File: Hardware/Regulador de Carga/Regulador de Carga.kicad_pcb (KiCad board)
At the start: 2 copper layers, 56 x 30 mm, 17 parts, among them Q1 2N3904

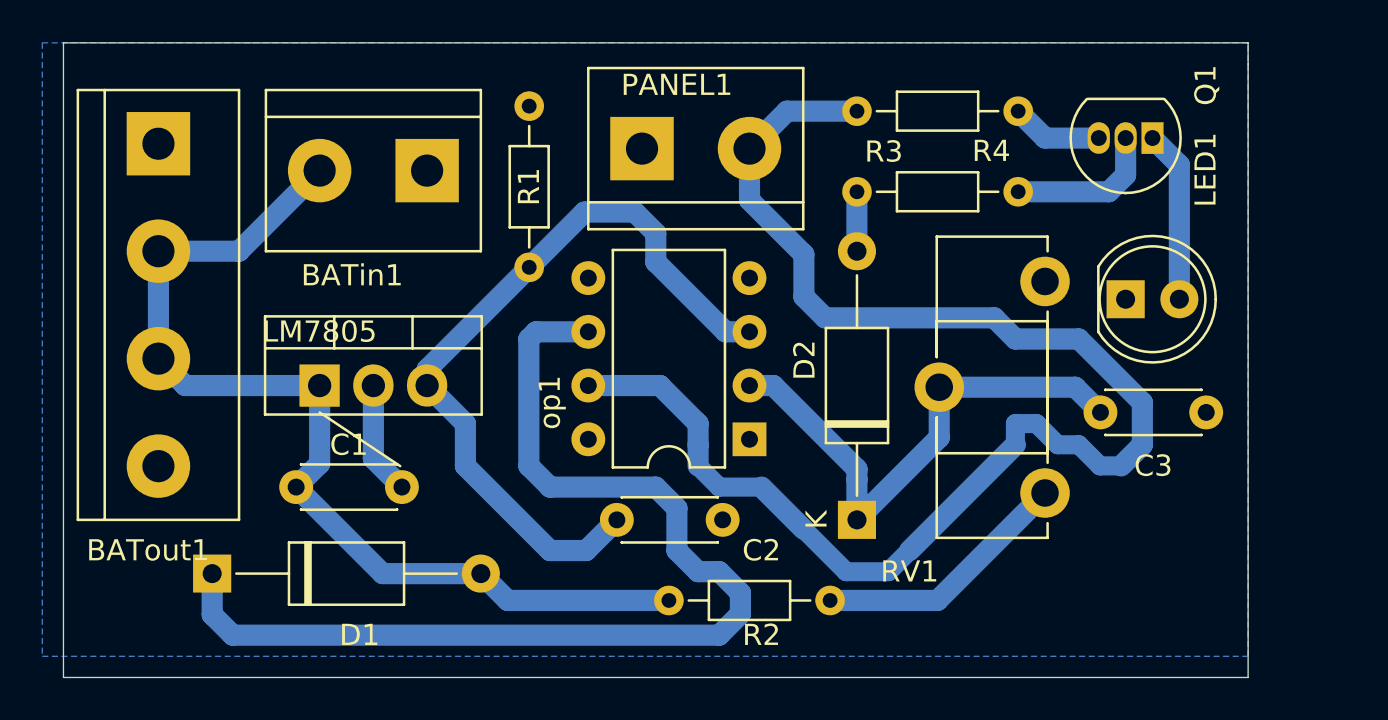
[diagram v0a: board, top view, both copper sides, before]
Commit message: PCB regulador de carga
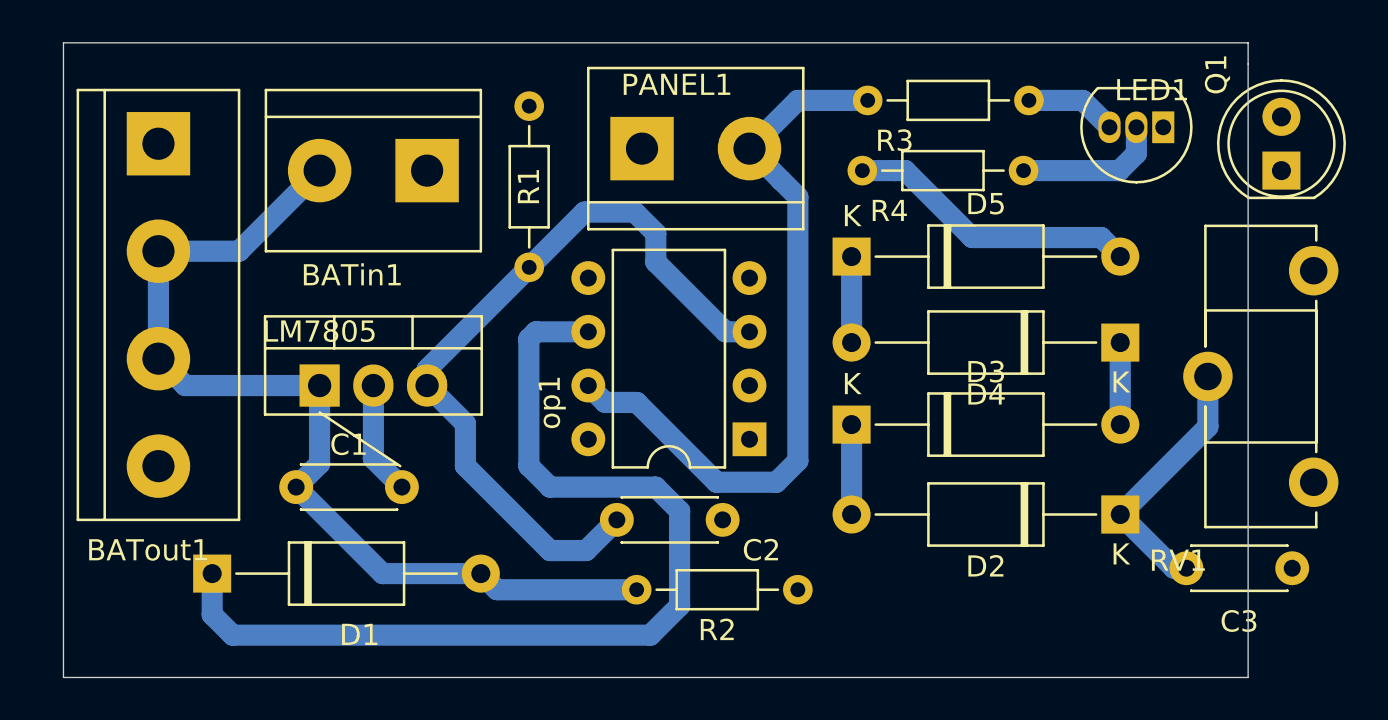
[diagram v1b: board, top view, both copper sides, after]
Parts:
- added D3: DIODE, Diode_THT:D_A-405_P12.70mm_Horizontal, F.Cu at (143.3, 78.0)
- added D4: DIODE, Diode_THT:D_A-405_P12.70mm_Horizontal, F.Cu at (156.0, 74.2)
- added D5: DIODE, Diode_THT:D_A-405_P12.70mm_Horizontal, F.Cu at (143.3, 70.1)
- D2: value D_Zener -> DIODE
- R3: value 1K -> 220
- R4: value 0K -> 220
- moved RV1 12.7 mm to (165.1, 80.8)
- moved D2 12.4 mm to (156.0, 82.3), turned to 180 degrees
- moved LED1 9.55 mm to (163.6, 66.0), turned to 90 degrees
- moved C3 8.41 mm to (164.1, 84.8)
- moved R4 7.94 mm to (151.4, 66.0), turned to 180 degrees
- moved R2 1.61 mm to (140.7, 85.9)
- moved Q1 0.72 mm to (158.0, 64.0)
- moved R3 0.72 mm to (151.6, 62.7)
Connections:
- D1 pad 1: (no net) -> Net-(D1-Pad1)
- R4 pad 1: Net-(D2-Pad2) -> Net-(Q1-Pad2)
- R4 pad 2: Net-(Q1-Pad2) -> Net-(D5-Pad2)
- op1 pad 2: Net-(C3-Pad2) -> Net-(op1-Pad2)
- op1 pad 6: (no net) -> Net-(D1-Pad1)
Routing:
- net (no net): track 51.3 -> 0.00 mm
- net Net-(D1-Pad1): track 0.00 -> 46.5 mm
- net Net-(PANEL1-Pad2): track 69.7 -> 34.5 mm
- net Net-(D5-Pad2): track 0.00 -> 13.9 mm
- net Net-(C3-Pad2): track 25.1 -> 12.4 mm
- net Net-(R2-Pad1): track 12.3 -> 0.00 mm
- net Net-(LED1-Pad2): track 8.15 -> 0.00 mm
- net Net-(D4-Pad2): track 0.00 -> 4.06 mm
- net Net-(D3-Pad2): track 0.00 -> 3.88 mm
- net Net-(BATin1-Pad2): track 47.5 -> 45.8 mm
- net Net-(D2-Pad2): track 2.81 -> 4.25 mm
- removed copper zone on B.Cu, net Earth
